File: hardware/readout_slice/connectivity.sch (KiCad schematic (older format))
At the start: 17 parts

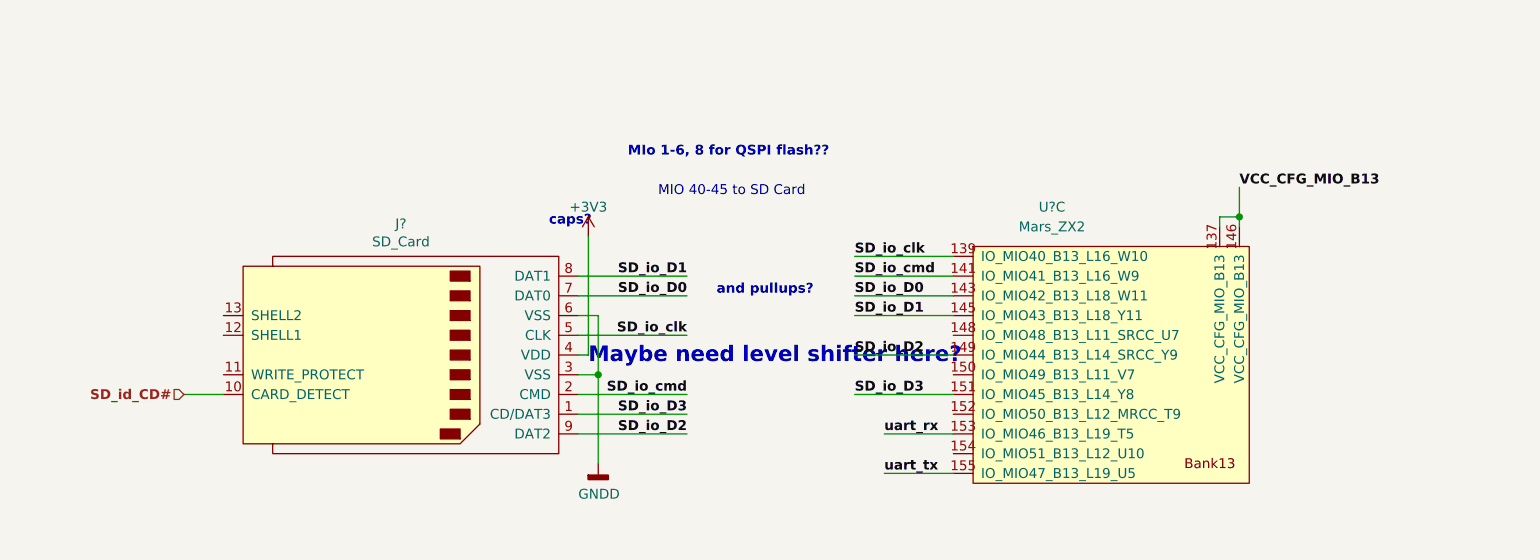
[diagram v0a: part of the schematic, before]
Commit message: auto push run at Mon Mar 15 12:11:48 EDT 2021
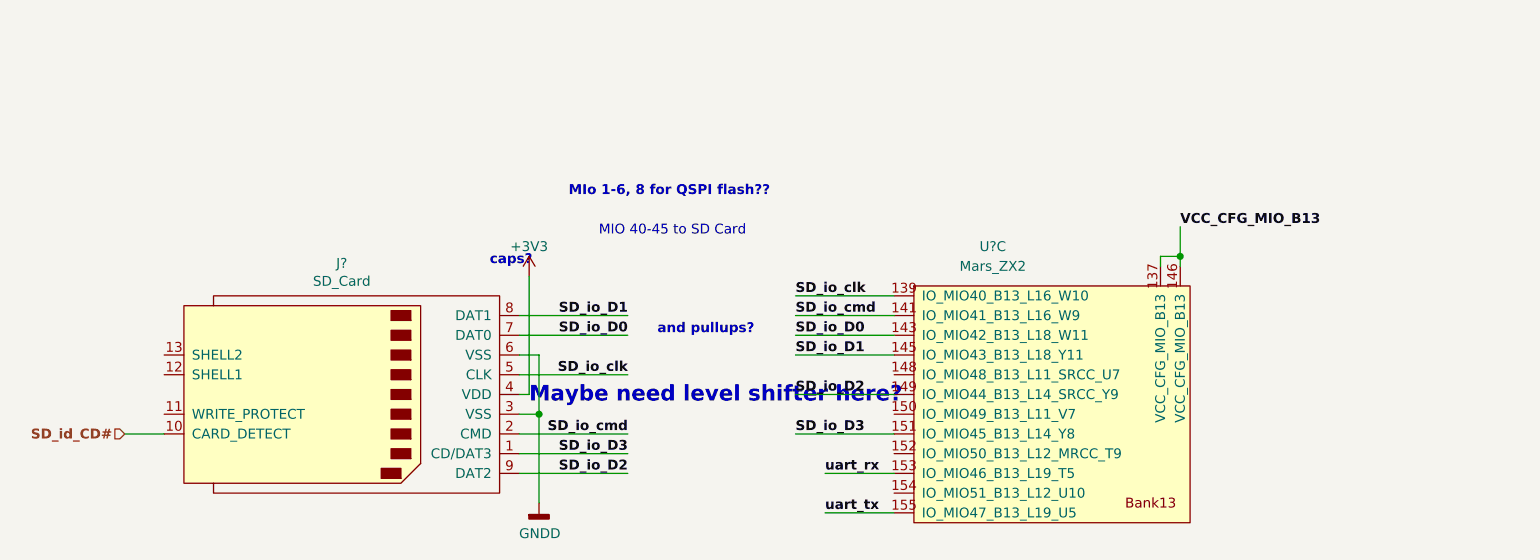
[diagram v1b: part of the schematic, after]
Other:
- moved on the sheet: J?, U?C
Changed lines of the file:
@@
 $Descr A4 11693 8268
 encoding utf-8
-Sheet 3 4
+Sheet 3 5
 Title ""
 Date ""
@@
 	8000 2200 7600 2200
 Wire Wire Line
-	5200 6250 4700 6250
-Wire Wire Line
-	4700 6350 5200 6350
-Wire Wire Line
-	4700 6450 5200 6450
-Wire Wire Line
-	4700 6550 5200 6550
-Wire Wire Line
-	4700 6750 5200 6750
-Wire Wire Line
-	4700 6950 5200 6950
-Text Notes 4450 5950 2    50   ~ 0
+	4900 6450 4400 6450
+Wire Wire Line
+	4400 6550 4900 6550
+Wire Wire Line
+	4400 6650 4900 6650
+Wire Wire Line
+	4400 6750 4900 6750
+Wire Wire Line
+	4400 6950 4900 6950
+Wire Wire Line
+	4400 7150 4900 7150
+Text Notes 4150 6150 2    50   ~ 0
 MIO 40-45 to SD Card
-Text Notes 3550 5750 0    50   ~ 10
+Text Notes 3250 5950 0    50   ~ 10
 MIo 1-6, 8 for QSPI flash??\n
 $Comp
 L Connector:SD_Card J?
 U 1 1 608C0AD2
-P 2400 6750
+P 2100 6950
 AR Path="/608C0AD2" Ref="J?"  Part="1"
 AR Path="/608B2FC0/608C0AD2" Ref="J?"  Part="1"
-F 0 "J?" H 2400 6085 50  0000 C CNN
-F 1 "SD_Card" H 2400 6176 50  0000 C CNN
-F 2 "" H 2400 6750 50  0001 C CNN
-F 3 "http://portal.fciconnect.com/Comergent//fci/drawing/10067847.pdf" H 2400 6750 50  0001 C CNN
-	1    2400 6750
+F 0 "J?" H 2100 6285 50  0000 C CNN
+F 1 "SD_Card" H 2100 6376 50  0000 C CNN
+F 2 "" H 2100 6950 50  0001 C CNN
+F 3 "http://portal.fciconnect.com/Comergent//fci/drawing/10067847.pdf" H 2100 6950 50  0001 C CNN
+	1    2100 6950
 	-1   0    0    1
 $EndComp
 Wire Wire Line
-	3300 6550 3400 6550
-Wire Wire Line
-	3400 6550 3400 6850
-Wire Wire Line
-	3300 6850 3400 6850
-Connection ~ 3400 6850
-Wire Wire Line
-	3400 6850 3400 7300
+	3000 6750 3100 6750
+Wire Wire Line
+	3100 6750 3100 7050
+Wire Wire Line
+	3000 7050 3100 7050
+Connection ~ 3100 7050
+Wire Wire Line
+	3100 7050 3100 7500
 $Comp
 L power:GNDD #PWR?
 U 1 1 608C0ADD
-P 3400 7300
+P 3100 7500
 AR Path="/608C0ADD" Ref="#PWR?"  Part="1"
 AR Path="/608B2FC0/608C0ADD" Ref="#PWR?"  Part="1"
-F 0 "#PWR?" H 3400 7050 50  0001 C CNN
-F 1 "GNDD" H 3404 7145 50  0000 C CNN
-F 2 "" H 3400 7300 50  0001 C CNN
-F 3 "" H 3400 7300 50  0001 C CNN
-	1    3400 7300
-	1    0    0    -1
-$EndComp
-Wire Wire Line
-	3300 6750 3350 6750
-Wire Wire Line
-	3350 6750 3350 6150
+F 0 "#PWR?" H 3100 7250 50  0001 C CNN
+F 1 "GNDD" H 3104 7345 50  0000 C CNN
+F 2 "" H 3100 7500 50  0001 C CNN
+F 3 "" H 3100 7500 50  0001 C CNN
+	1    3100 7500
+	1    0    0    -1
+$EndComp
+Wire Wire Line
+	3000 6950 3050 6950
+Wire Wire Line
+	3050 6950 3050 6350
 $Comp
 L power:+3V3 #PWR?
 U 1 1 608C0AE5
-P 3350 6150
+P 3050 6350
 AR Path="/608C0AE5" Ref="#PWR?"  Part="1"
 AR Path="/608B2FC0/608C0AE5" Ref="#PWR?"  Part="1"
-F 0 "#PWR?" H 3350 6000 50  0001 C CNN
-F 1 "+3V3" H 3350 6300 50  0000 C CNN
-F 2 "" H 3350 6150 50  0001 C CNN
-F 3 "" H 3350 6150 50  0001 C CNN
-	1    3350 6150
-	1    0    0    -1
-$EndComp
-Text Notes 3150 6100 0    50   ~ 10
+F 0 "#PWR?" H 3050 6200 50  0001 C CNN
+F 1 "+3V3" H 3050 6500 50  0000 C CNN
+F 2 "" H 3050 6350 50  0001 C CNN
+F 3 "" H 3050 6350 50  0001 C CNN
+	1    3050 6350
+	1    0    0    -1
+$EndComp
+Text Notes 2850 6300 0    50   ~ 10
 caps?
 $Comp
 L readout:Mars_ZX2 U?
 U 3 1 608C0AEC
-P 5700 6100
+P 5400 6300
 AR Path="/608C0AEC" Ref="U?"  Part="3"
 AR Path="/608B2FC0/608C0AEC" Ref="U?"  Part="3"
-F 0 "U?" H 5700 6200 50  0000 C CNN
-F 1 "Mars_ZX2" H 5700 6100 50  0000 C CNN
-F 2 "" H 5750 6450 50  0001 C CNN
-F 3 "" H 5750 6450 50  0001 C CNN
-	3    5700 6100
+F 0 "U?" H 5400 6400 50  0000 C CNN
+F 1 "Mars_ZX2" H 5400 6300 50  0000 C CNN
+F 2 "" H 5450 6650 50  0001 C CNN
+F 3 "" H 5450 6650 50  0001 C CNN
+	3    5400 6300
 	-1   0    0    -1
 $EndComp
@@
 $EndComp
 Wire Wire Line
-	5200 7150 4850 7150
-Wire Wire Line
-	5200 7350 4850 7350
-Text Label 4850 7150 0    50   ~ 10
+	4900 7350 4550 7350
+Wire Wire Line
+	4900 7550 4550 7550
+Text Label 4550 7350 0    50   ~ 10
 uart_rx
-Text Label 4850 7350 0    50   ~ 10
+Text Label 4550 7550 0    50   ~ 10
 uart_tx
 $Comp
@@
 	-1   0    0    1
 $EndComp
-Text Label 6650 5900 0    50   ~ 10
+Text Label 6350 6100 0    50   ~ 10
 VCC_CFG_MIO_B13
 Wire Wire Line
-	6650 5900 6650 6050
-Wire Wire Line
-	6650 6050 6550 6050
-Wire Wire Line
-	6550 6050 6550 6100
-Connection ~ 6650 6050
-Wire Wire Line
-	6650 6050 6650 6100
-Text Label 4700 6250 0    50   ~ 10
+	6350 6100 6350 6250
+Wire Wire Line
+	6350 6250 6250 6250
+Wire Wire Line
+	6250 6250 6250 6300
+Connection ~ 6350 6250
+Wire Wire Line
+	6350 6250 6350 6300
+Text Label 4400 6450 0    50   ~ 10
 SD_io_clk
-Text Label 4700 6350 0    50   ~ 10
+Text Label 4400 6550 0    50   ~ 10
 SD_io_cmd
-Text Label 4700 6450 0    50   ~ 10
+Text Label 4400 6650 0    50   ~ 10
 SD_io_D0
-Text Label 4700 6550 0    50   ~ 10
+Text Label 4400 6750 0    50   ~ 10
 SD_io_D1
-Text Label 4700 6750 0    50   ~ 10
+Text Label 4400 6950 0    50   ~ 10
 SD_io_D2
-Text Label 4700 6950 0    50   ~ 10
+Text Label 4400 7150 0    50   ~ 10
 SD_io_D3
-Text Label 3850 7150 2    50   ~ 10
+Text Label 3550 7350 2    50   ~ 10
 SD_io_D2
 Wire Wire Line
-	3850 7150 3300 7150
-Text Label 3850 7050 2    50   ~ 10
+	3550 7350 3000 7350
+Text Label 3550 7250 2    50   ~ 10
 SD_io_D3
 Wire Wire Line
-	3850 7050 3300 7050
-Text Label 3850 6950 2    50   ~ 10
+	3550 7250 3000 7250
+Text Label 3550 7150 2    50   ~ 10
 SD_io_cmd
 Wire Wire Line
-	3850 6950 3300 6950
-Text Label 3850 6650 2    50   ~ 10
+	3550 7150 3000 7150
+Text Label 3550 6850 2    50   ~ 10
 SD_io_clk
 Wire Wire Line
-	3850 6650 3300 6650
-Text Label 3850 6450 2    50   ~ 10
+	3550 6850 3000 6850
+Text Label 3550 6650 2    50   ~ 10
 SD_io_D0
 Wire Wire Line
-	3850 6450 3300 6450
-Text Label 3850 6350 2    50   ~ 10
+	3550 6650 3000 6650
+Text Label 3550 6550 2    50   ~ 10
 SD_io_D1
 Wire Wire Line
-	3850 6350 3300 6350
-Wire Wire Line
-	1300 6950 1500 6950
+	3550 6550 3000 6550
+Wire Wire Line
+	1000 7150 1200 7150
 NoConn ~ 11050 6350
 NoConn ~ 11050 6250
@@
 Text HLabel 6550 2600 2    50   Input ~ 0
 PS_SRST
-Text HLabel 1300 6950 0    50   Input ~ 10
+Text HLabel 1000 7150 0    50   Input ~ 10
 SD_id_CD#
-Text Notes 3350 6800 0    79   ~ 16
+Text Notes 3050 7000 0    79   ~ 16
 Maybe need level shifter here?
 $Comp
@@
 Text HLabel 4000 2350 2    50   Input ~ 10
 Vcc_0
-Text Notes 4000 6450 0    50   ~ 10
+Text Notes 3700 6650 0    50   ~ 10
 and pullups?\n
 $EndSCHEMATC
